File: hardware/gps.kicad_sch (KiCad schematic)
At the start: 10 parts, among them J23 OCXO Volt, J6 GPS ANT, J7 GPS Module, U5 TXS0108EPW, U7 NEO-M8M, U8 DAC8571IDGK

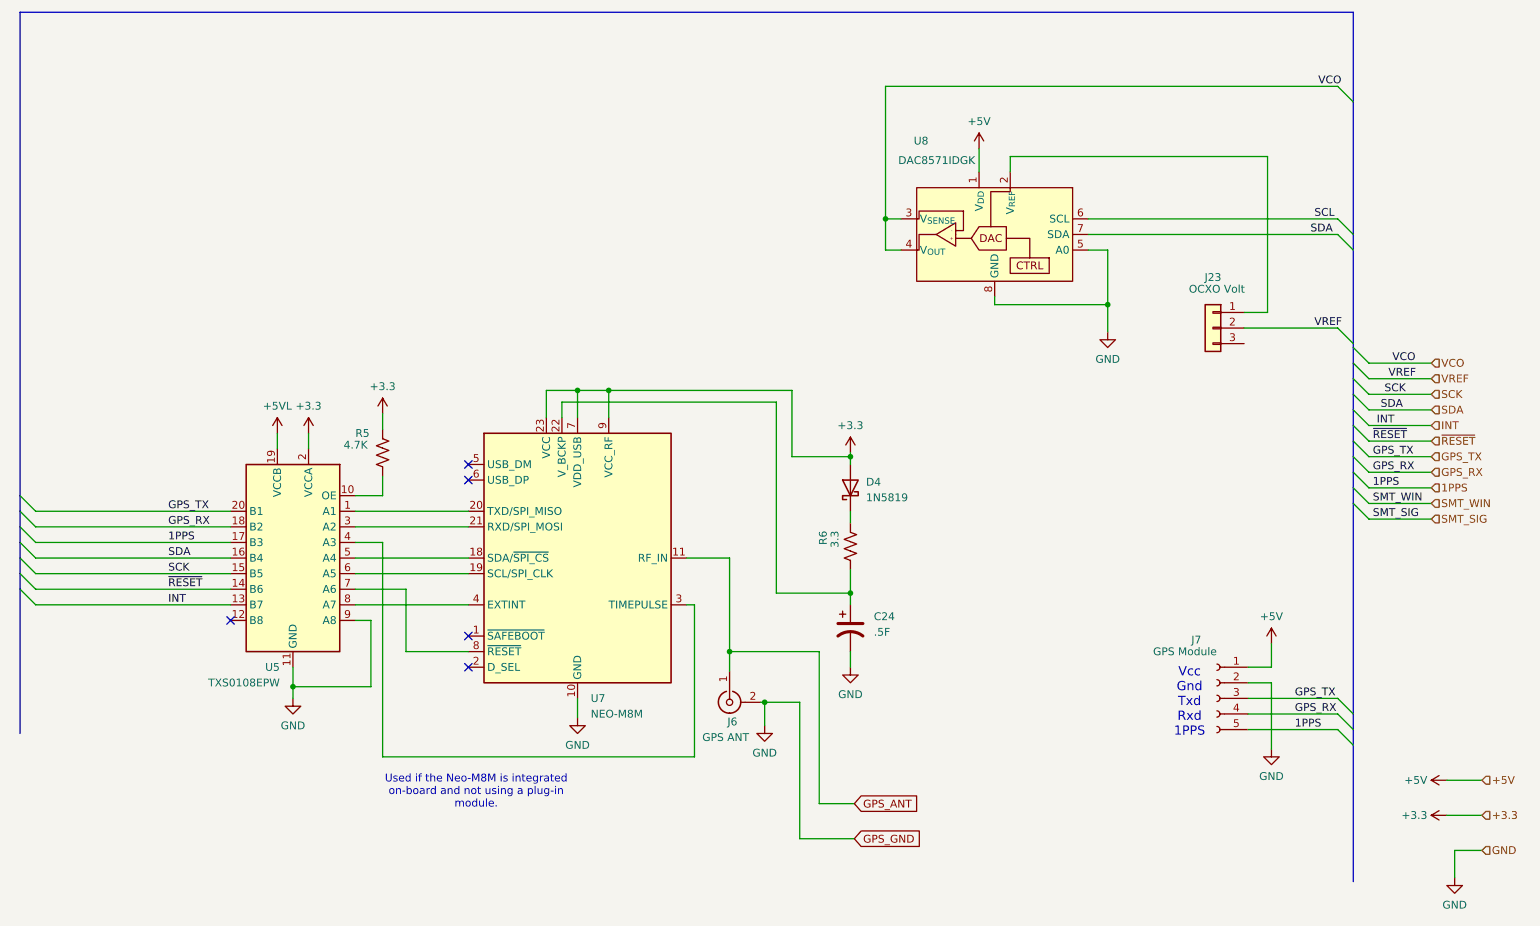
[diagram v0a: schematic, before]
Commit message: Revised hardware design
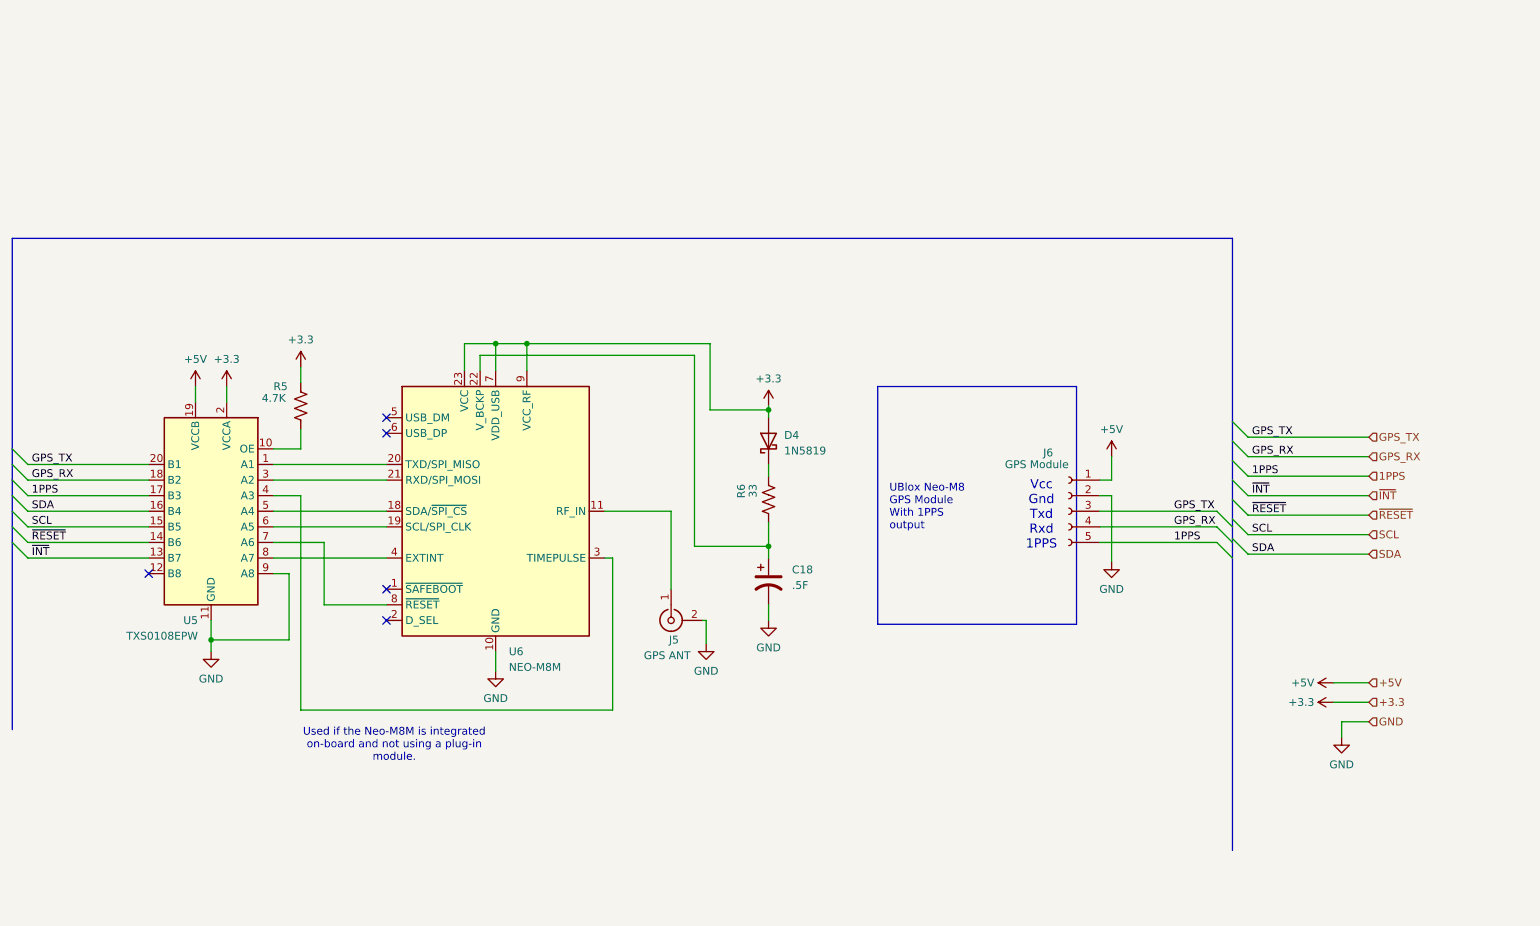
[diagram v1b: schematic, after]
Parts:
- removed J23: OCXO Volt, symbol Connector_Generic:Conn_01x03
- removed U8: DAC8571IDGK, Package_SO:MSOP-8_3x3mm_P0.65mm, symbol Analog_DAC:DAC8571IDGK
- R6: value 3.3 -> 33
- renumbered C24 to C18, J6 to J5, J7 to J6, U7 to U6
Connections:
- net +5VL is gone; now on net +5V: U5.19 (VCCB)
- net SCK is gone; now on net SCL: U5.15 (B5)
- net GPS_ANT: no longer names the net of J5.1 (In), U6.11 (RF_IN)
- net INT renamed ~{INT}
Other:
- note added: "UBlox Neo-M8 GPS Module With 1PPS output"
- moved on the sheet: C18, D4, J5, J6, R5, R6, U5, U6
